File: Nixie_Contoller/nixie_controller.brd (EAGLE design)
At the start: 111.7 x 49.2 mm, 28 parts, among them IC1 DS1307, IC2 7805TV, J1 CON-SOCJ-2155, Q1 16MHz, U1 328P, U2 HU2032-LF, Y2 32.768kHz

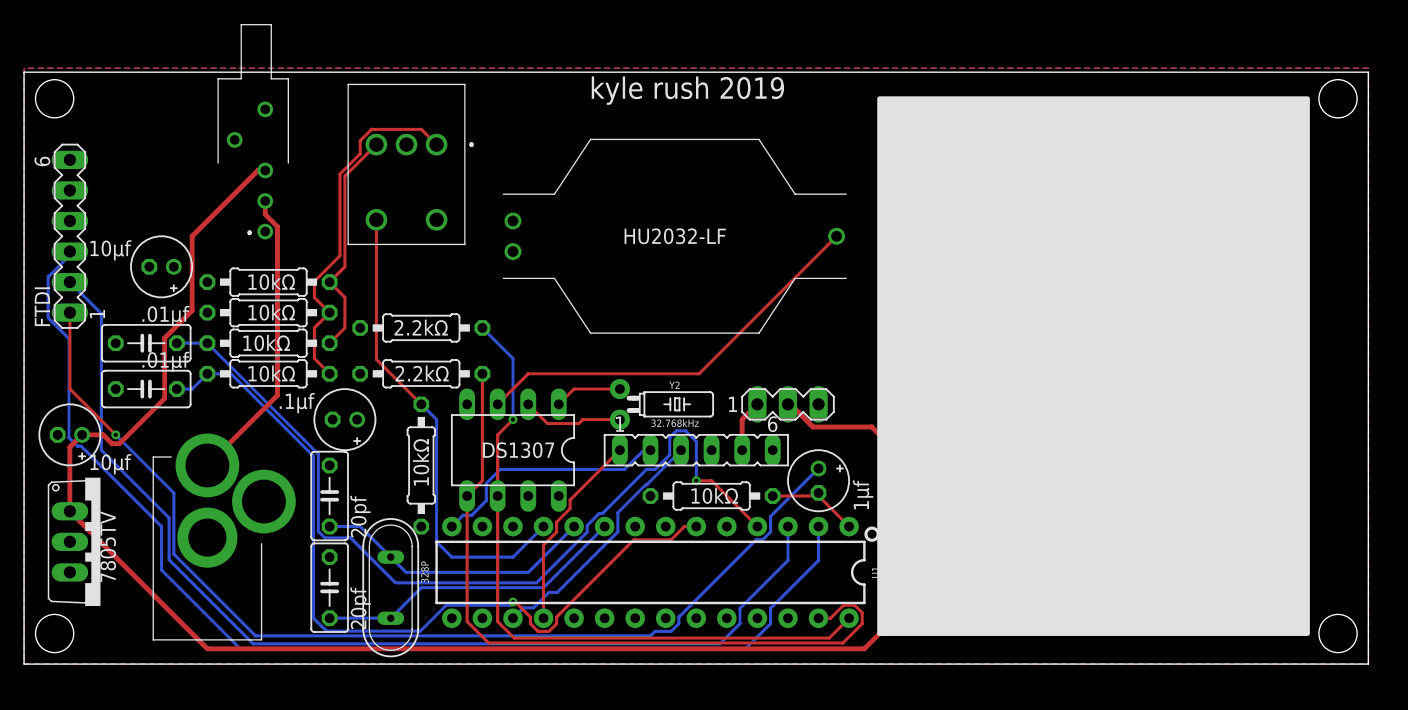
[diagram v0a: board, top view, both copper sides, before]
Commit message: Snapshot 12-23
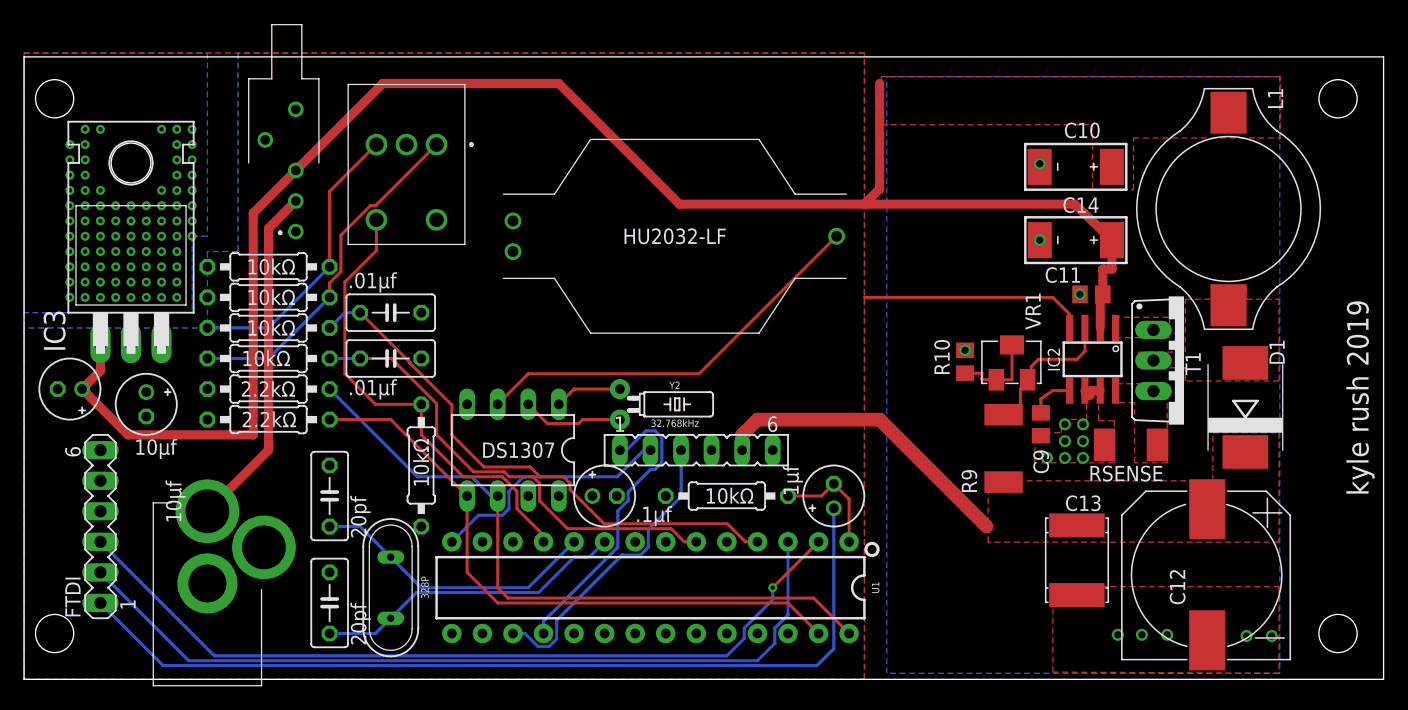
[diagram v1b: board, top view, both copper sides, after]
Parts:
- removed SV2: (no value), con-lstb:MA03-1
- added C10: 100uF,35V, nick:C-EIA-7343
- added C11, C9: 100n, rcl:C0805
- added C12: 4u7,250V, nick:NICHICON-UJ-12
- added C13: 100n,250V, nick:C2420
- added C14: 10uF,25V, nick:C-EIA-7343
- added D1: ES2F, diode:SMC
- added IC3: 7805T, linear:TO220H
- added L1: 100uH, nick:L-B82479
- added R10: 10K, rcl:R0805
- added R9: 1M5, rcl:R2512
- added RSENSE: 0R050, rcl:R2010
- added T1: IRF644PBF, transistor-power:TO220BV
- added VR1: 5K, nick:BOURNS-3214W
- IC2: value 7805TV -> MAX1771ESA; device linear:TO220V -> nick:SO-8
- moved IC2 83.9 mm to (88.8, 25.3), turned to 180 degrees
- moved FTDI 24.3 mm to (6.35, 11.4)
- moved C5 22.5 mm to (48.3, 14.0), turned to 0 degrees
- moved C3 20.5 mm to (30.5, 29.2), turned to 0 degrees
- moved C4 20.5 mm to (30.5, 25.4), turned to 0 degrees
- moved R1 13.7 mm to (20.3, 22.9)
- moved R2 13.3 mm to (20.3, 20.3)
- moved C2 11.5 mm to (10.2, 21.6), turned to 270 degrees
- moved J1 3.81 mm to (15.2, 12.7)
- moved C1 3.81 mm to (3.81, 22.9)
- moved S2 2.54 mm to (21.6, 44.5)
- moved C8 1.80 mm to (67.3, 14.0), turned to 90 degrees
- moved R3 1.27 mm to (20.3, 33.0)
- moved R8 1.27 mm to (58.4, 14.0)
- moved U1 1.27 mm to (52.1, 6.35)
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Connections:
- new net EXT: IC2.1, T1.G
- new net N$19: D1.A, L1.P$2, T1.D
- new net N$20: C9.1, IC2.5
- new net N$23: R10.2, VR1.1, VR1.2
- new net N$24: IC2.8, RSENSE.2, T1.S
- new net N$8: IC2.3, R9.1, VR1.3
- net +12V: now also C10.+, C11.1, C14.+, IC2.2, IC3.1, L1.P$1; no longer IC2.1, SV2.2
- net GND: now also C10.-, C11.2, C12.1, C13.P$2, C14.-, C9.2, IC2.4, IC2.6, IC2.7, IC3.2, R10.1, RSENSE.1; no longer IC2.2, SV2.3
- net V+: now also C12.2, C13.P$1, D1.C, R9.2; no longer SV2.1
- net VCC: now also IC3.3; no longer IC2.3
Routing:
- net N$10: track 66.7 -> 39.2 mm, vias 1 -> 0
- net N$22: track 95.2 -> 68.6 mm, vias 0 -> 1
- net N$9: track 71.9 -> 45.8 mm, vias 1 -> 0
- net V+: track 4.34 -> 25.8 mm
- net GND: track 0.00 -> 20.4 mm, vias 0 -> 97
- net N$21: track 87.3 -> 68.6 mm
- net N$8: track 0.00 -> 12.2 mm
- net N$17: track 86.9 -> 75.4 mm, vias 1 -> 0
- net N$13: track 60.6 -> 51.7 mm
- net CLK: track 16.6 -> 25.0 mm
- net N$23: track 0.00 -> 7.35 mm
- net N$18: track 20.7 -> 26.0 mm
- net N$15: track 19.3 -> 24.0 mm
- net N$6: track 24.8 -> 28.8 mm
- net N$20: track 0.00 -> 3.77 mm
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- added copper zone on layer 1, net +12V
- added copper zone on layer 1, net EXT
- added copper zone on layer 16, net GND
- added copper zone on layer 1, net N$19
- added copper zone on layer 1, net N$24
- added copper zone on layer 1, net V+
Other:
- board size 111.7 x 49.2 mm -> 113 x 51.7 mm
- board text added: "0.000"
- board text added: "0.001"
- board text added: "0.146"
- board text added: "0.154"
- board text added: "1.209"
- board text added: "1.508"
- board text added: "1.512"
- board text added: "1.655"
- board text added: "1.839"
- board text added: "2.026"
